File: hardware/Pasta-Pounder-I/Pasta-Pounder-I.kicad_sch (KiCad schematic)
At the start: 62 parts, among them CN1 XT30UPB-M, CN2 B4B-PH-K-S(LF)(SN), J1 USB_C_Receptacle, J2 Brushed_Motor_1, J3 Brushed_Motor_2, J4 ESC_Port, J5 Flipper_port, J6 ESC_Terminal, Q1 AO3401A, SW1 RESET-SW, SW2 BOOT-SW, SW3 5.8 ZSPT, U1 DRV8874PWPR, U2 DRV8874PWPR, U4 USBLC6-2P6, U5 ESP32S3W1, U6 SY8113BADC, U7 SY8113BADC

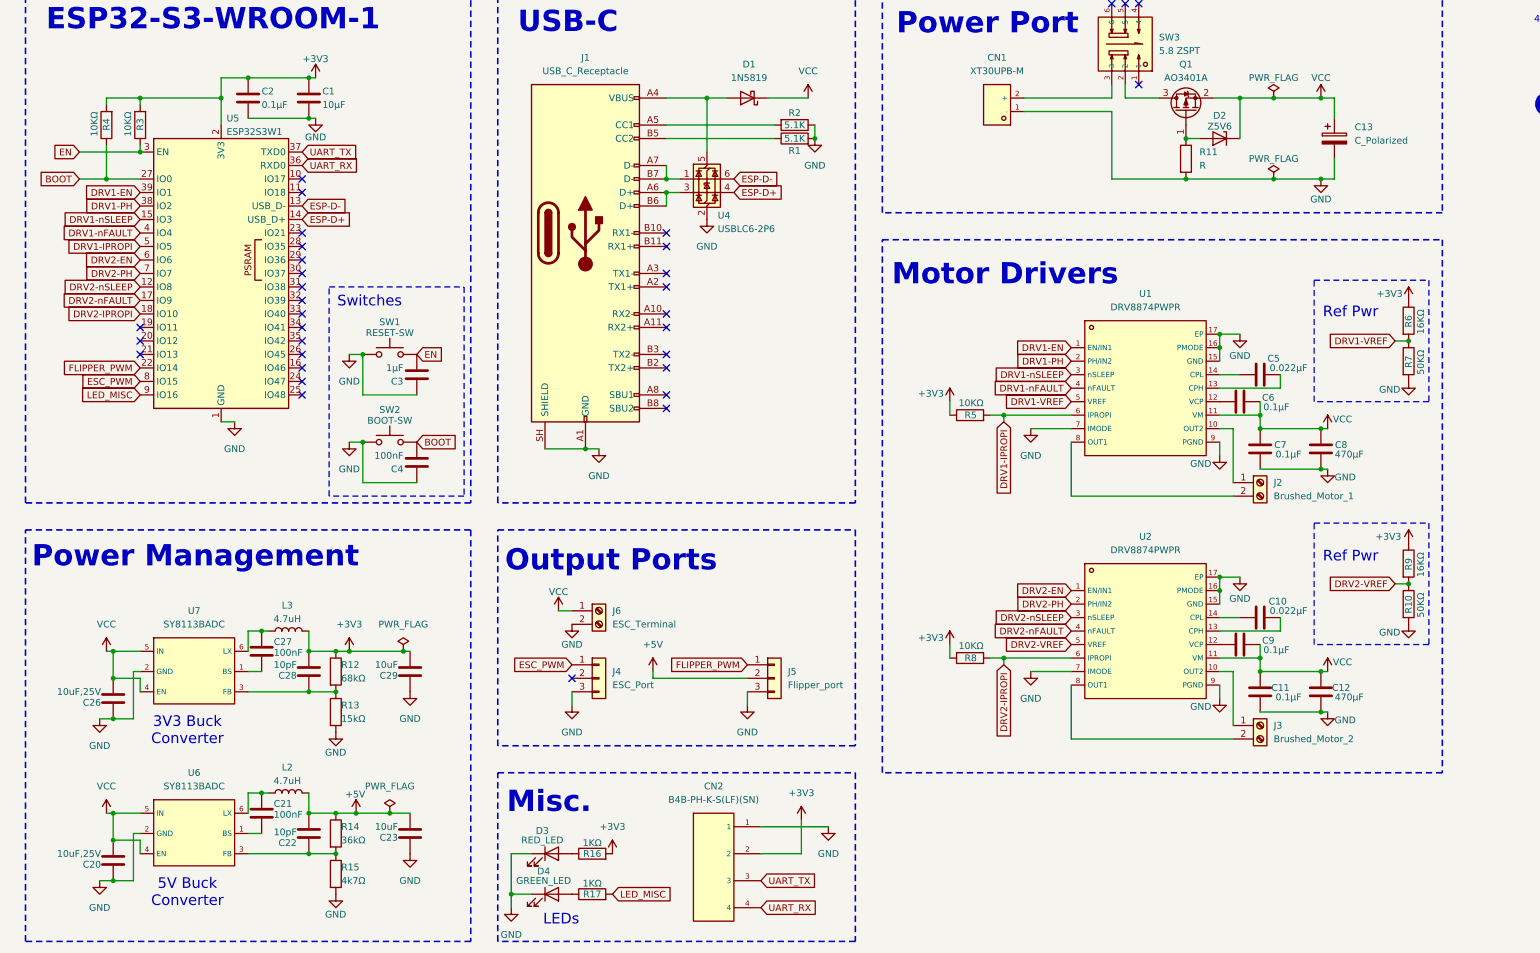
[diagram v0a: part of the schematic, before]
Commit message: Fixed minor issues for schematic freeze
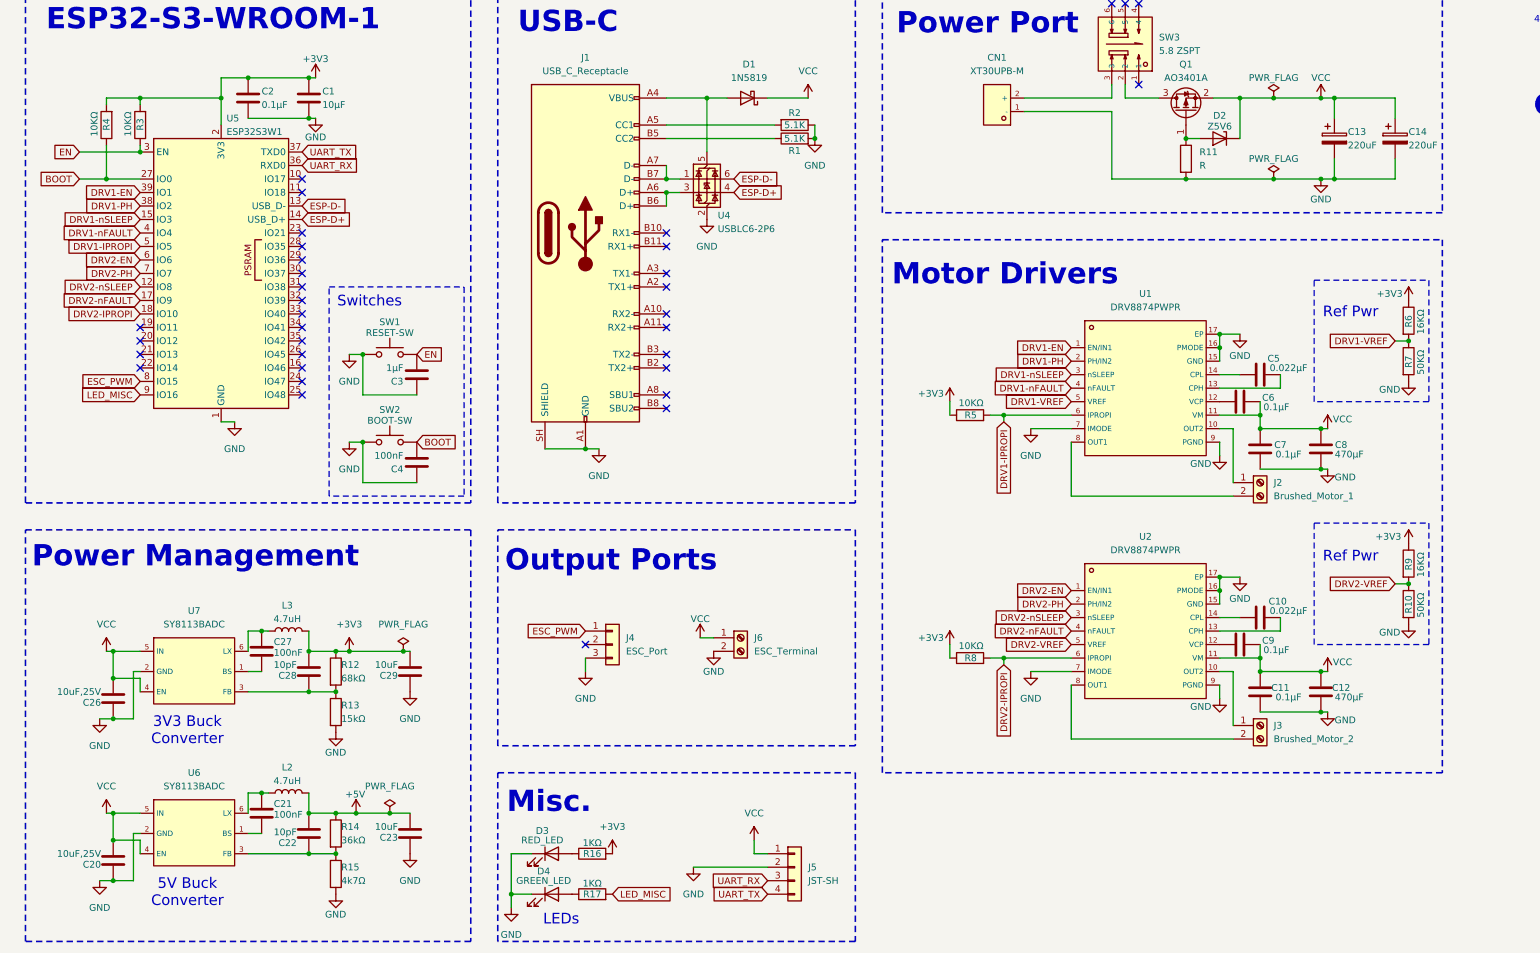
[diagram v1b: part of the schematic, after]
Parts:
- removed CN2: B4B-PH-K-S(LF)(SN), lcsc_footprints:C131334_CONN-TH_B4B-PH-K-S, symbol lcsc_imported:B4B-PH-K-S(LF)(SN)
- removed J5: Flipper_port, symbol Connector_Generic:Conn_01x03
- added C14: 220uF, symbol Device:C_Polarized
- added J5: JST-SH, symbol Connector_Generic:Conn_01x04
- C13: value C_Polarized -> 220uF
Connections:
- net GND: now also C14.2, J5.2 (Pin_2)
- net UART_RX: now also J5.3 (Pin_3)
- net UART_TX: now also J5.4 (Pin_4)
- net VCC: now also C14.1, J5.1 (Pin_1)
- net FLIPPER_PWM: no longer names the net of U5.22 (IO14)
- no-connect marks 33 -> 34
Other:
- moved on the sheet: J4, J6
